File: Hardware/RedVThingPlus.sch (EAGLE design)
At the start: 83 parts, among them J1 FEMALE 2x3, J2 USB Female Type C Connector, J5 JTAG, Q1 3.1A/30V/105mΩ, U1 MCP73831, U2 1.8V, U3 AP2112-3.3V, U4 FE310, U5 32MB, Y1 32.768KHZ, Y2 16MHz

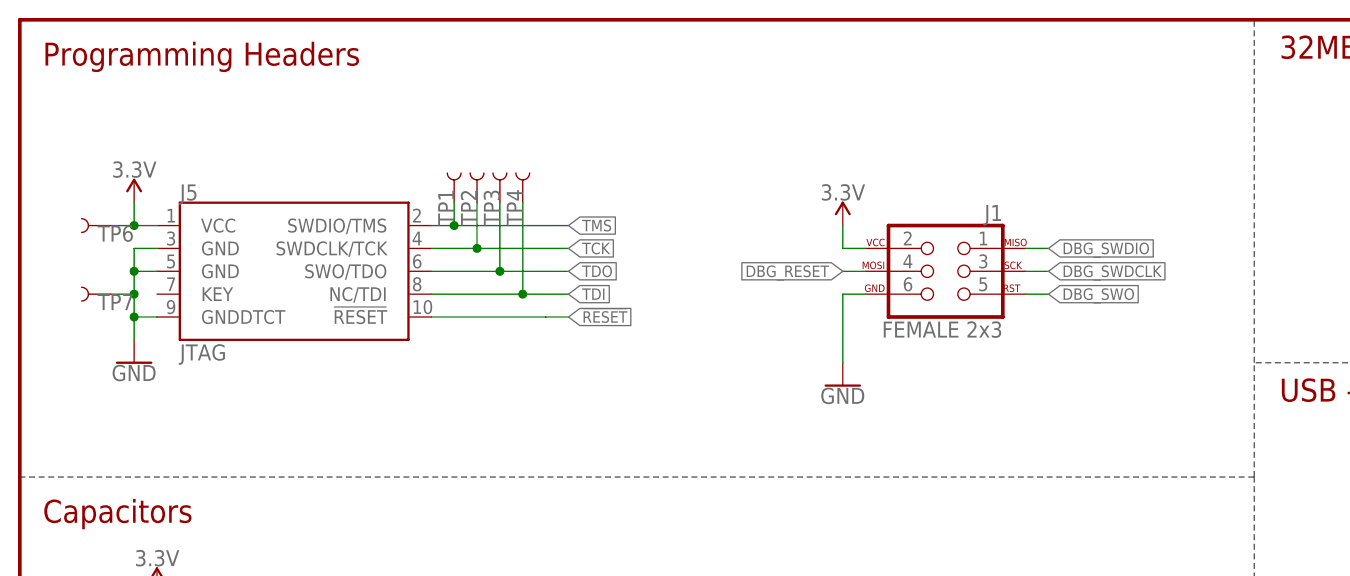
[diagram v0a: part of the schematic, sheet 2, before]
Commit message: initial layout complete, needs silk
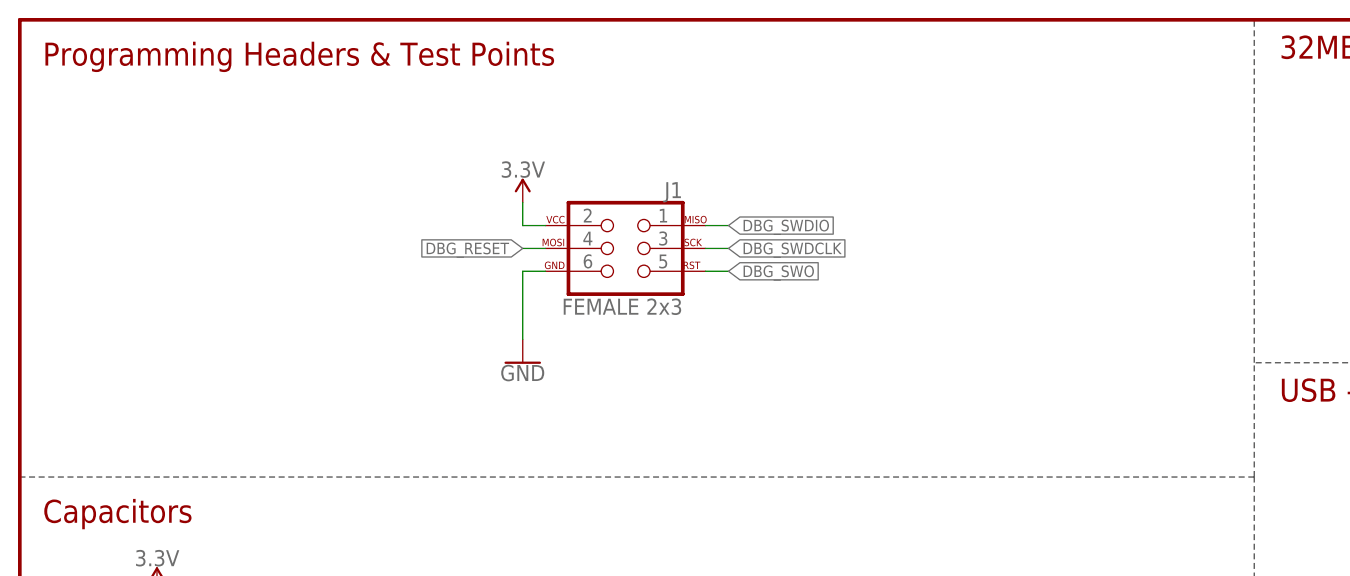
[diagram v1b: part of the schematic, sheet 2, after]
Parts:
- removed J5: JTAG, SparkFun-Connectors:CORTEX_JTAG_DEBUG_SMD
- removed TP1, TP2, TP3, TP4, TP6, TP7: TEST-POINT3, SparkFun-Connectors:TEST-POINT3
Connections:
- net !RESET: no longer J5.!RESET
- net 3.3V: no longer J5.VCC, TP6.1
- net GND: no longer J5.GND@3, J5.GND@5, J5.GNDDTCT, TP7.1
- net TCK: no longer J5.SWDCLK/TCK, TP2.1
- net TDI: no longer J5.NC/TDI, TP4.1
- net TDO: no longer J5.SWO/TDO, TP3.1
- net TMS: no longer J5.SWDIO/TMS, TP1.1
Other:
- note added: "Programming Headers & Test Points"
- note removed: "Programming Headers"
- moved on the sheet: J1
